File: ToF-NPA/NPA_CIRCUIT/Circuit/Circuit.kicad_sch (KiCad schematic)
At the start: 10 parts, among them J1 BG302-02-A-L-G

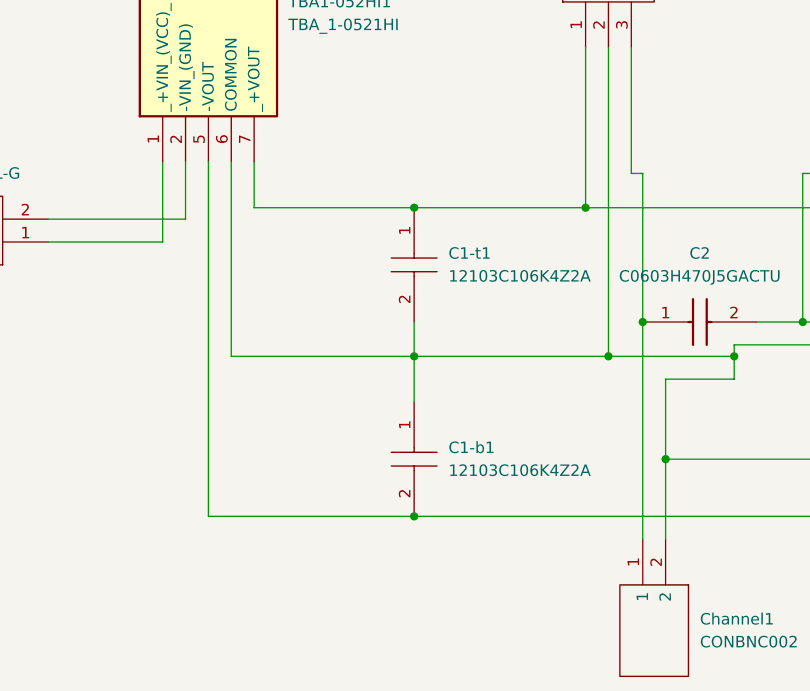
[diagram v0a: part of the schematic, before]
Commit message: now we're done
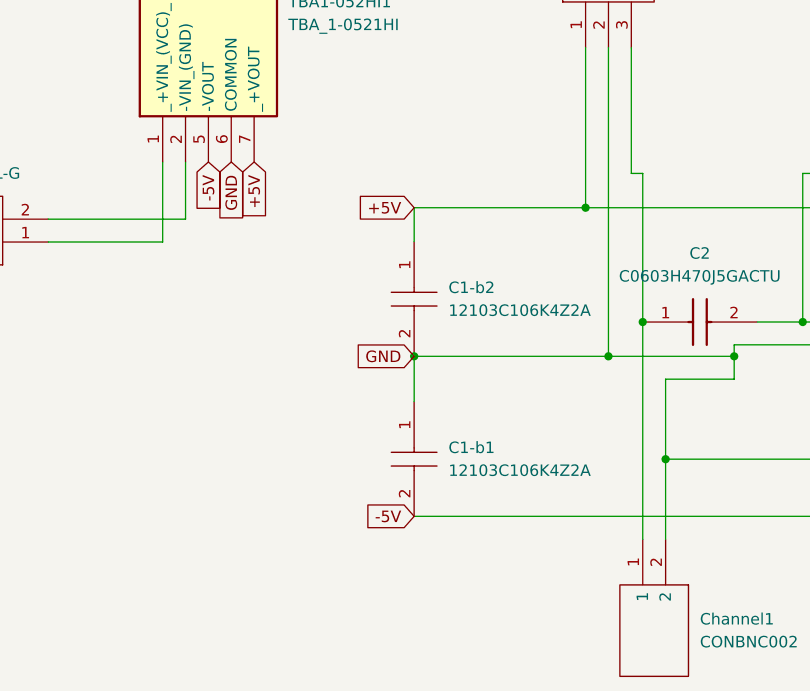
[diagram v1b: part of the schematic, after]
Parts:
- removed C1-t1: 12103C106K4Z2A, CAPC3225X279N, symbol 12103C106K4Z2A:12103C106K4Z2A
- added C1-b2: 12103C106K4Z2A, CAPC3225X279N, symbol 12103C106K4Z2A:12103C106K4Z2A
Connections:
- net GND: now reaches C1-b1.1, Channel1.2, Channel2.2, OpAmp1.3 (+IN), TBA1-052HI1.6 (COMMON), brown-blue-white1.2
- net GND: now also C1-b2.2
- net -5V: now reaches C1-b1.2, OpAmp1.4 (V-), TBA1-052HI1.5 (-VOUT)
- net +5V: now reaches OpAmp1.7 (V+), TBA1-052HI1.7 (_+VOUT), brown-blue-white1.1
- net +5V: now also C1-b2.1
